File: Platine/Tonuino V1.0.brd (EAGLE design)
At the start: 81 x 50 mm, 32 parts, among them T1 BC857, T2 BC847, T3 BC847, T4 IRLML2502

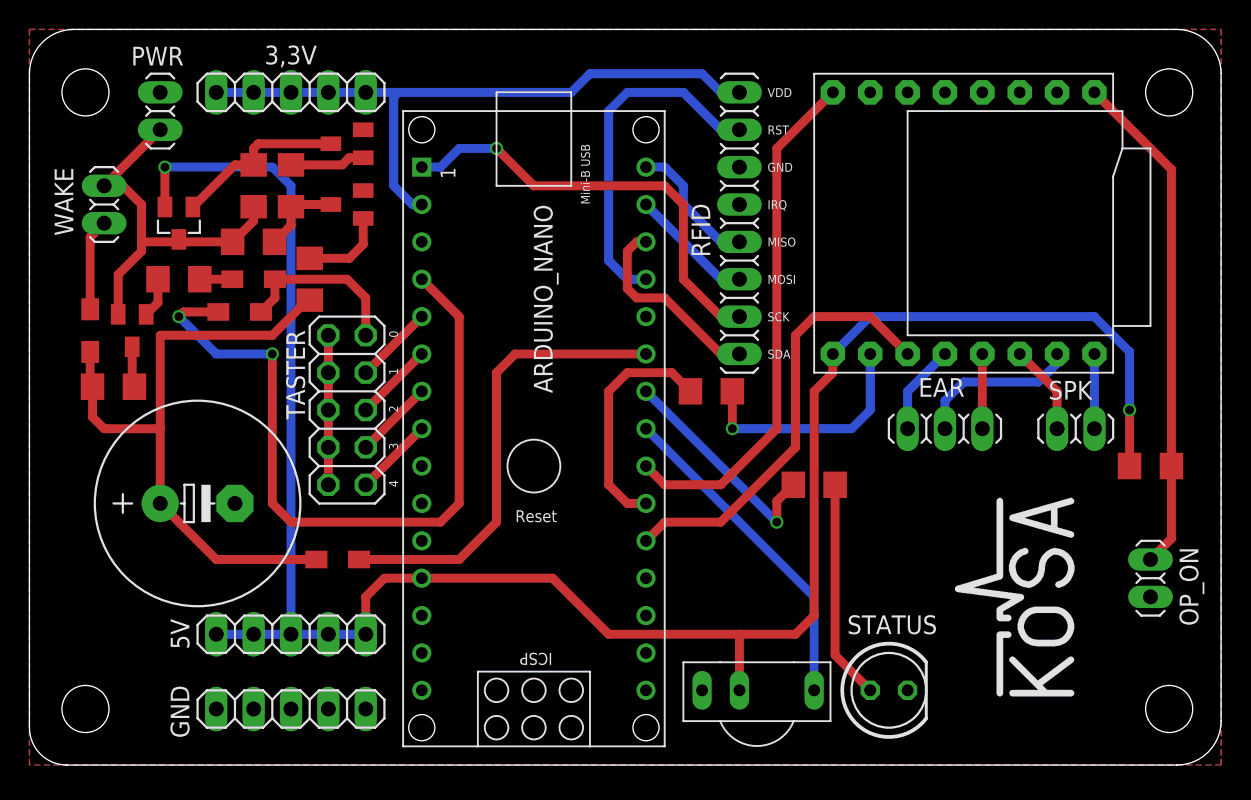
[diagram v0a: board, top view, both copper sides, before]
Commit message: Add files via upload
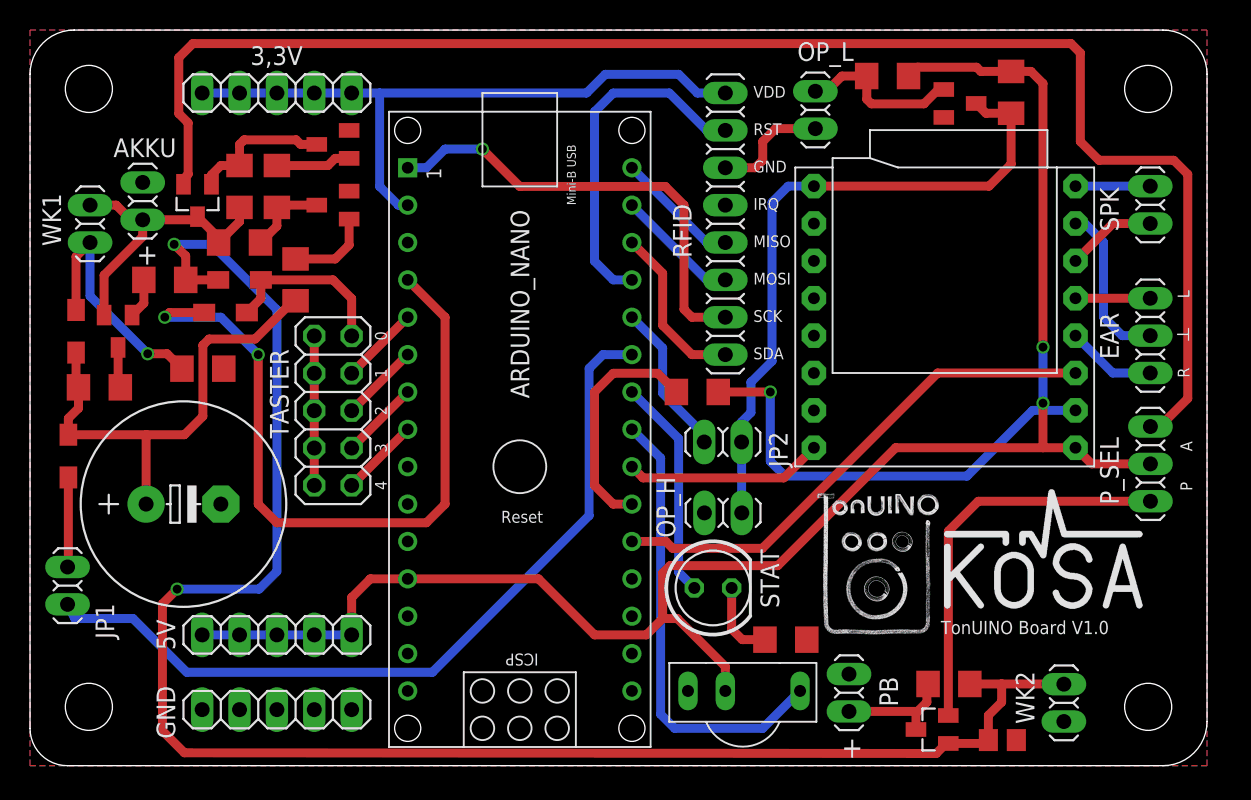
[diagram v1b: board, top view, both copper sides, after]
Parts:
- removed OP_ON, PWR, WAKE: (no value), pinhead:1X02
- removed STATUS: (no value), led:LED5MM
- added AKKU, JP1, JP2, OP_H, OP_L, PB, WK1, WK2: (no value), pinhead:1X02
- added C2: 33n, rcl:C0805
- added P_SEL: (no value), pinhead:1X03
- added R10: 100, rcl:R1206
- added R11: 3M, rcl:R1206
- added R12: 2,5k, rcl:R1206
- added STAT: (no value), led:LED5MM
- added T5: IRLML2502, transistor-fet:SOT23
- added T6: BC847, transistor:SOT23
- C1: value (none) -> 220µF
- moved R7 27.1 mm to (66.7, 45.7), turned to 270 degrees
- moved D2 19.6 mm to (2.65, 21.0), turned to 270 degrees
- moved SPK 16.0 mm to (76.2, 38.1), turned to 270 degrees
- moved EAR 15.3 mm to (76.2, 29.2), turned to 270 degrees
- moved R8 10.7 mm to (51.4, 8.52)
- moved U$2 6.50 mm to (62.2, 30.5), turned to 180 degrees
- moved T4 2.00 mm to (11.4, 38.4)
- moved 3,3V 0.96 mm to (16.8, 45.7)
- moved 5V 0.96 mm to (16.8, 8.85)
- moved GND 0.96 mm to (16.8, 3.77)
- moved R9 0.96 mm to (18.1, 33.0)
- moved R5 0.96 mm to (16.8, 39.3)
- moved D1 0.96 mm to (3.17, 29.5)
- moved C1 0.96 mm to (10.5, 17.7)
- moved D3 0.96 mm to (14.3, 33.0)
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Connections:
- new net N$16: R8.2, STAT.K
- new net N$17: ARDUINO_NANO.26, JP2.1
- new net N$20: PB.2, R11.2, T5.3
- new net PWR_ON_PIN_JPR: ARDUINO_NANO.25, JP1.1
- new net VCC_AKKU: P_SEL.3, T4.2
- new net VCC_PB: P_SEL.1, T5.2
- net GND: now also AKKU.1, C2.2, OP_H.1, OP_L.1, PB.1, R10.1, R8.1, T6.2, WK2.1; no longer OP_ON.1, PWR.1, STATUS.K
- net N$10: now also JP2.2, OP_H.2, T6.3; no longer OP_ON.2
- net N$22: now also STAT.A; no longer R8.2
- net N$23: now also OP_L.2, R12.2, T6.1; no longer R8.1, STATUS.A
- net N$25: now also R10.2, WK1.1; no longer WAKE.1
- net PWR_ON_PIN: now also JP1.2; no longer ARDUINO_NANO.25
- net TASTER: now also C2.1, R11.1, T5.1, WK2.2
- net VCC: now also AKKU.2, WK1.2; no longer PWR.2, WAKE.2
- net VCC_TONUINO: now also P_SEL.2, R12.1; no longer T4.2
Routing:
- net TASTER: track 2.21 -> 116.6 mm, vias 0 -> 2
- net VCC_AKKU: track 0.00 -> 103.8 mm
- net PWR_ON_PIN_JPR: track 0.00 -> 55.3 mm
- net VCC_PB: track 0.00 -> 27.1 mm
- net PWR_ON_PIN: track 31.2 -> 6.14 mm
- net N$9: track 35.4 -> 13.5 mm
- net VCC_TONUINO: track 140.2 -> 118.5 mm
- net N$6: track 16.2 -> 31.3 mm
- net N$24: track 44.2 -> 32.7 mm
- net N$10: track 34.5 -> 45.4 mm
- net N$25: track 6.25 -> 16.9 mm, vias 0 -> 1
- net N$17: track 0.00 -> 10.5 mm
- net N$21: track 22.5 -> 31.1 mm
- net N$20: track 0.00 -> 8.09 mm
- net GND: track 10.2 -> 18.1 mm
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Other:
- board size 81 x 50 mm -> 80 x 50 mm
- board text added: "+"
- board text added: "A"
- board text added: "L"
- board text added: "P"
- board text added: "R"
- board text added: "TonUINO Board V1.0"
